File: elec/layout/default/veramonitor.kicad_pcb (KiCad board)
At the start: 2 copper layers, 55 parts, among them J1 ?, U1 ?, U10 ?, U11 ?, U12 ?, U13 ?, U14 ?, U15 ?, U16 ?, U17 ?, U18 ?, U19 ?, U2 ?, U20 ?, U21 ?, U22 ?, U23 ?, U24 ?, U25 ?, U26 ?, U3 ?, U4 ?, U5 ?, U6 ?, U7 ?, U8 ?, U9 ?

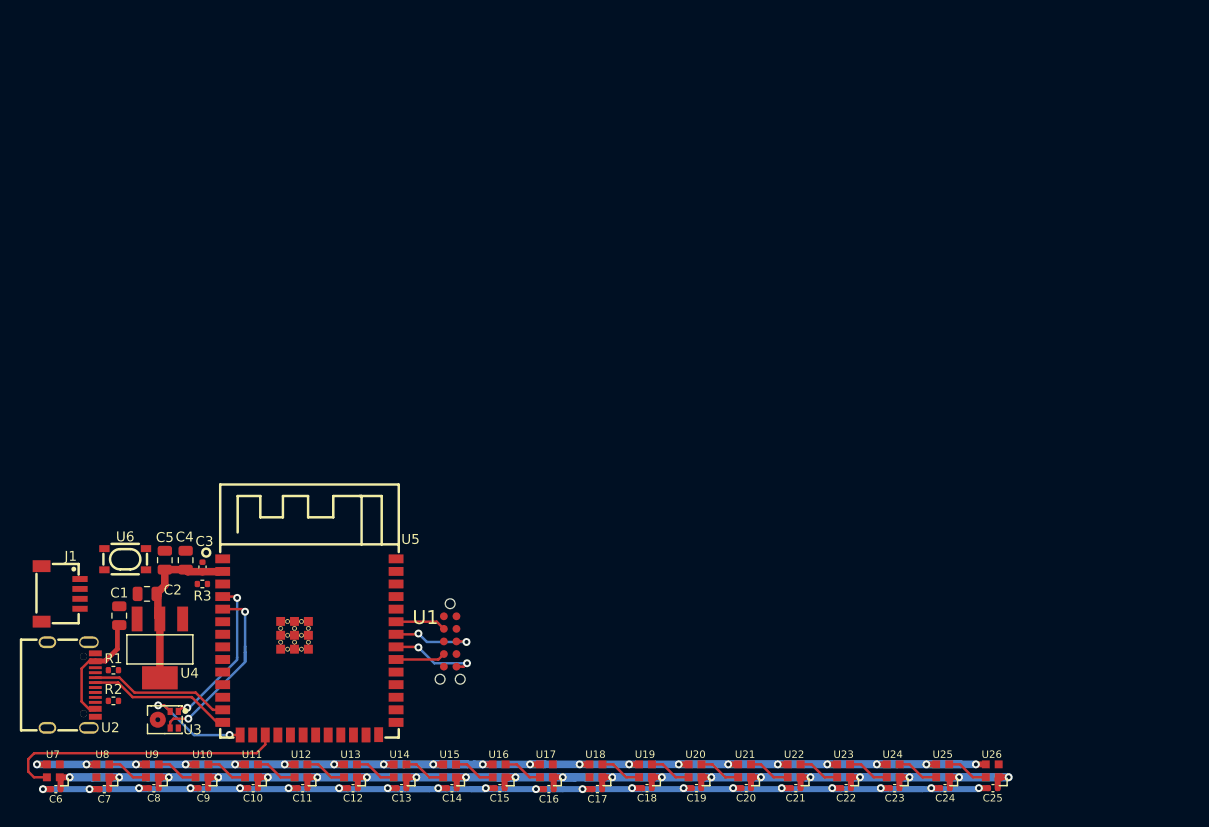
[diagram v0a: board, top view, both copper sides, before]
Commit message: eod 10/30
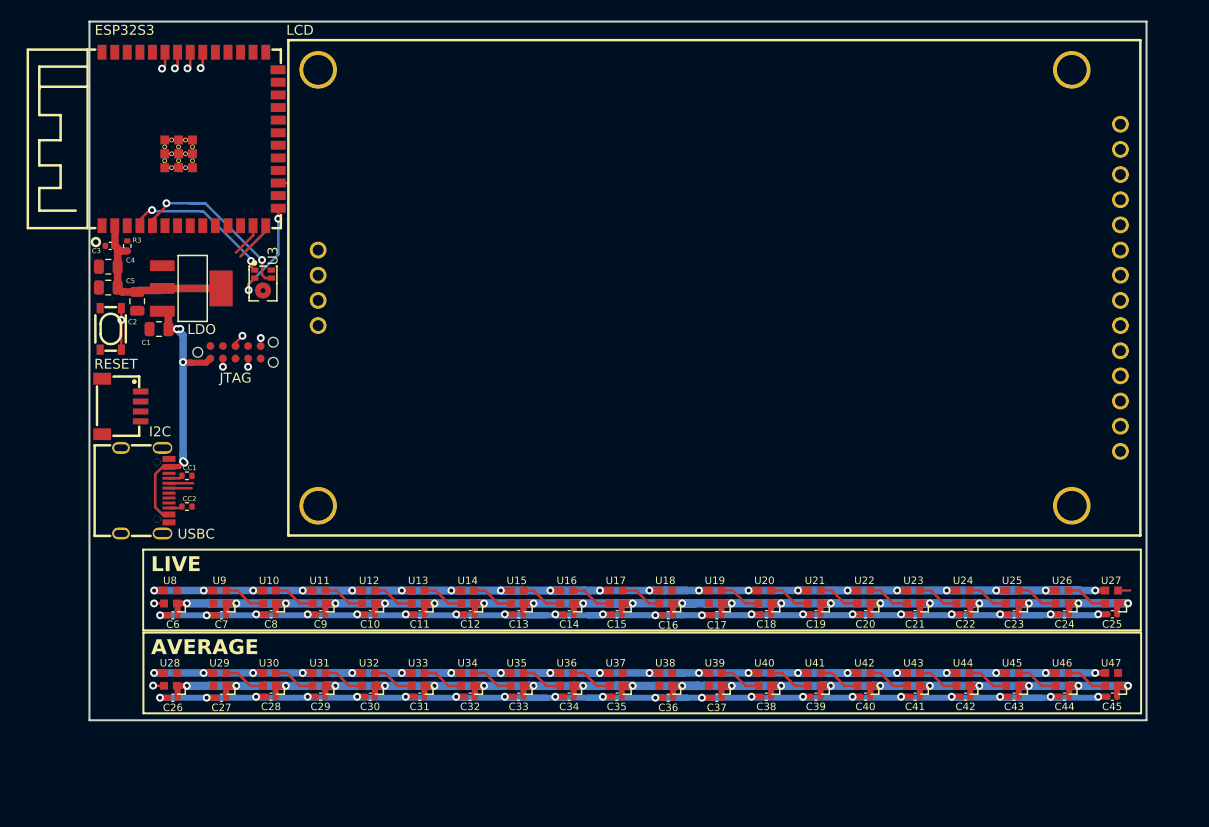
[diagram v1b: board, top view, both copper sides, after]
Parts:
- added C26: 16V 100nF X7R ±10% 0402 Multilayer Ceramic Capacitors MLCC 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, lib:C0402, F.Cu at (48.8, 135.2)
- added C27: 16V 100nF X7R ±10% 0402 Multilayer Ceramic Capacitors MLCC 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, lib:C0402, F.Cu at (53.7, 135.2)
- added C28: 16V 100nF X7R ±10% 0402 Multilayer Ceramic Capacitors MLCC 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, lib:C0402, F.Cu at (58.7, 135.1)
- added C29: 16V 100nF X7R ±10% 0402 Multilayer Ceramic Capacitors MLCC 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, lib:C0402, F.Cu at (63.7, 135.1)
- added C30: 16V 100nF X7R ±10% 0402 Multilayer Ceramic Capacitors MLCC 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, lib:C0402, F.Cu at (68.7, 135.1)
- added C31: 16V 100nF X7R ±10% 0402 Multilayer Ceramic Capacitors MLCC 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, lib:C0402, F.Cu at (73.7, 135.1)
- added C32: 16V 100nF X7R ±10% 0402 Multilayer Ceramic Capacitors MLCC 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, lib:C0402, F.Cu at (78.8, 135.1)
- added C33: 16V 100nF X7R ±10% 0402 Multilayer Ceramic Capacitors MLCC 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, lib:C0402, F.Cu at (83.7, 135.1)
- added C34: 16V 100nF X7R ±10% 0402 Multilayer Ceramic Capacitors MLCC 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, lib:C0402, F.Cu at (88.8, 135.1)
- added C35: 16V 100nF X7R ±10% 0402 Multilayer Ceramic Capacitors MLCC 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, lib:C0402, F.Cu at (93.6, 135.1)
- added C36: 16V 100nF X7R ±10% 0402 Multilayer Ceramic Capacitors MLCC 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, lib:C0402, F.Cu at (98.8, 135.2)
- added C37: 16V 100nF X7R ±10% 0402 Multilayer Ceramic Capacitors MLCC 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, lib:C0402, F.Cu at (103.7, 135.2)
- added C38: 16V 100nF X7R ±10% 0402 Multilayer Ceramic Capacitors MLCC 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, lib:C0402, F.Cu at (108.7, 135.1)
- added C39: 16V 100nF X7R ±10% 0402 Multilayer Ceramic Capacitors MLCC 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, lib:C0402, F.Cu at (113.7, 135.1)
- added C40: 16V 100nF X7R ±10% 0402 Multilayer Ceramic Capacitors MLCC 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, lib:C0402, F.Cu at (118.7, 135.1)
- added C41: 16V 100nF X7R ±10% 0402 Multilayer Ceramic Capacitors MLCC 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, lib:C0402, F.Cu at (123.7, 135.1)
- added C42: 16V 100nF X7R ±10% 0402 Multilayer Ceramic Capacitors MLCC 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, lib:C0402, F.Cu at (128.8, 135.1)
- added C43: 16V 100nF X7R ±10% 0402 Multilayer Ceramic Capacitors MLCC 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, lib:C0402, F.Cu at (133.7, 135.1)
- added C44: 16V 100nF X7R ±10% 0402 Multilayer Ceramic Capacitors MLCC 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, lib:C0402, F.Cu at (138.8, 135.1)
- added C45: 16V 100nF X7R ±10% 0402 Multilayer Ceramic Capacitors MLCC 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, lib:C0402, F.Cu at (143.6, 135.1)
- added LCD: ?, lib:COMM-TH_HS12864G18B, F.Cu at (103.9, 93.8)
- added U28: ?, lib:LED-SMD_4P-L2.0-W2.0-BR, F.Cu at (48.5, 133.4)
- added U29: ?, lib:LED-SMD_4P-L2.0-W2.0-BR, F.Cu at (53.5, 133.4)
- added U30: ?, lib:LED-SMD_4P-L2.0-W2.0-BR, F.Cu at (58.5, 133.4)
- added U31: ?, lib:LED-SMD_4P-L2.0-W2.0-BR, F.Cu at (63.5, 133.4)
- added U32: ?, lib:LED-SMD_4P-L2.0-W2.0-BR, F.Cu at (68.5, 133.4)
- added U33: ?, lib:LED-SMD_4P-L2.0-W2.0-BR, F.Cu at (73.5, 133.4)
- added U34: ?, lib:LED-SMD_4P-L2.0-W2.0-BR, F.Cu at (78.5, 133.4)
- added U35: ?, lib:LED-SMD_4P-L2.0-W2.0-BR, F.Cu at (83.5, 133.4)
- added U36: ?, lib:LED-SMD_4P-L2.0-W2.0-BR, F.Cu at (88.5, 133.4)
- added U37: ?, lib:LED-SMD_4P-L2.0-W2.0-BR, F.Cu at (93.5, 133.4)
- added U38: ?, lib:LED-SMD_4P-L2.0-W2.0-BR, F.Cu at (98.5, 133.4)
- added U39: ?, lib:LED-SMD_4P-L2.0-W2.0-BR, F.Cu at (103.5, 133.4)
- added U40: ?, lib:LED-SMD_4P-L2.0-W2.0-BR, F.Cu at (108.5, 133.4)
- added U41: ?, lib:LED-SMD_4P-L2.0-W2.0-BR, F.Cu at (113.5, 133.4)
- added U42: ?, lib:LED-SMD_4P-L2.0-W2.0-BR, F.Cu at (118.5, 133.4)
- added U43: ?, lib:LED-SMD_4P-L2.0-W2.0-BR, F.Cu at (123.5, 133.4)
- added U44: ?, lib:LED-SMD_4P-L2.0-W2.0-BR, F.Cu at (128.5, 133.4)
- added U45: ?, lib:LED-SMD_4P-L2.0-W2.0-BR, F.Cu at (133.5, 133.4)
- added U46: ?, lib:LED-SMD_4P-L2.0-W2.0-BR, F.Cu at (138.5, 133.4)
- added U47: ?, lib:LED-SMD_4P-L2.0-W2.0-BR, F.Cu at (143.5, 133.4)
- moved ESP32S3 52.7 mm to (50.5, 78.8), turned to 90 degrees
- moved U3 45.2 mm to (57.9, 93.3), turned to 0 degrees
- moved LDO 36.5 mm to (50.7, 93.9), turned to 180 degrees
- moved JTAG 36.3 mm to (55.1, 100.4), turned to 0 degrees
- moved R3 35.0 mm to (44.2, 89.6), turned to 90 degrees
- moved C3 33.7 mm to (42.5, 89.6), turned to 180 degrees
- moved C4 30.6 mm to (42.2, 91.7), turned to 180 degrees
- moved C2 29.5 mm to (45.2, 95.2), turned to -90 degrees
- moved C1 29.2 mm to (47.4, 98.0), turned to 180 degrees
- moved C5 28.1 mm to (42.2, 93.8), turned to 180 degrees
- moved RESET 23.3 mm to (42.5, 98.0), turned to -90 degrees
- moved C22 21.3 mm to (128.8, 126.8)
- moved C23 21.3 mm to (133.7, 126.8)
- moved C25 21.3 mm to (143.6, 126.8)
- moved U18 21.3 mm to (98.5, 125.0)
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- renumbered R1 to CC1, R2 to CC2, U5 to ESP32S3, J1 to I2C, U1 to JTAG, U4 to LDO, U6 to RESET, U9 to U10, U10 to U11, U11 to U12, U12 to U13, U13 to U14, U14 to U15, U15 to U16, U16 to U17, U17 to U18, U18 to U19, U19 to U20, U20 to U21, U21 to U22, U22 to U23, U23 to U24, U24 to U25, U25 to U26, U26 to U27, U7 to U8, U8 to U9, U2 to USBC
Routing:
- net gnd: track 314.7 -> 636.1 mm, vias 40 -> 80
- net vcc: track 176.0 -> 349.7 mm, vias 20 -> 45
- net led_data: track 28.9 -> 1.97 mm, vias 0 -> 1
- net dm: track 14.2 -> 5.88 mm
- net dp: track 14.5 -> 6.47 mm
- net tdo: track 9.05 -> 2.55 mm
- net tdi: track 8.60 -> 3.16 mm
- net ledrow4.led6.ic-vcc: track 0.00 -> 4.24 mm
- net ledrow4.led5.ic-vcc: track 0.00 -> 4.24 mm
- net ledrow4.led4.ic-vcc: track 0.00 -> 4.24 mm
- net ledrow4.led3.ic-vcc: track 0.00 -> 4.24 mm
- net ledrow4.led2.ic-vcc: track 0.00 -> 4.24 mm
- net ledrow3.led9.ic-vcc: track 0.00 -> 4.24 mm
- net ledrow3.led8.ic-vcc: track 0.00 -> 4.24 mm
- net ledrow3.led7.ic-vcc: track 0.00 -> 4.24 mm
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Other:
- board outline added: 106.7 x 70.5 mm
- board text added: "AVERAGE"
- board text added: "LIVE"

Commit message: finished?
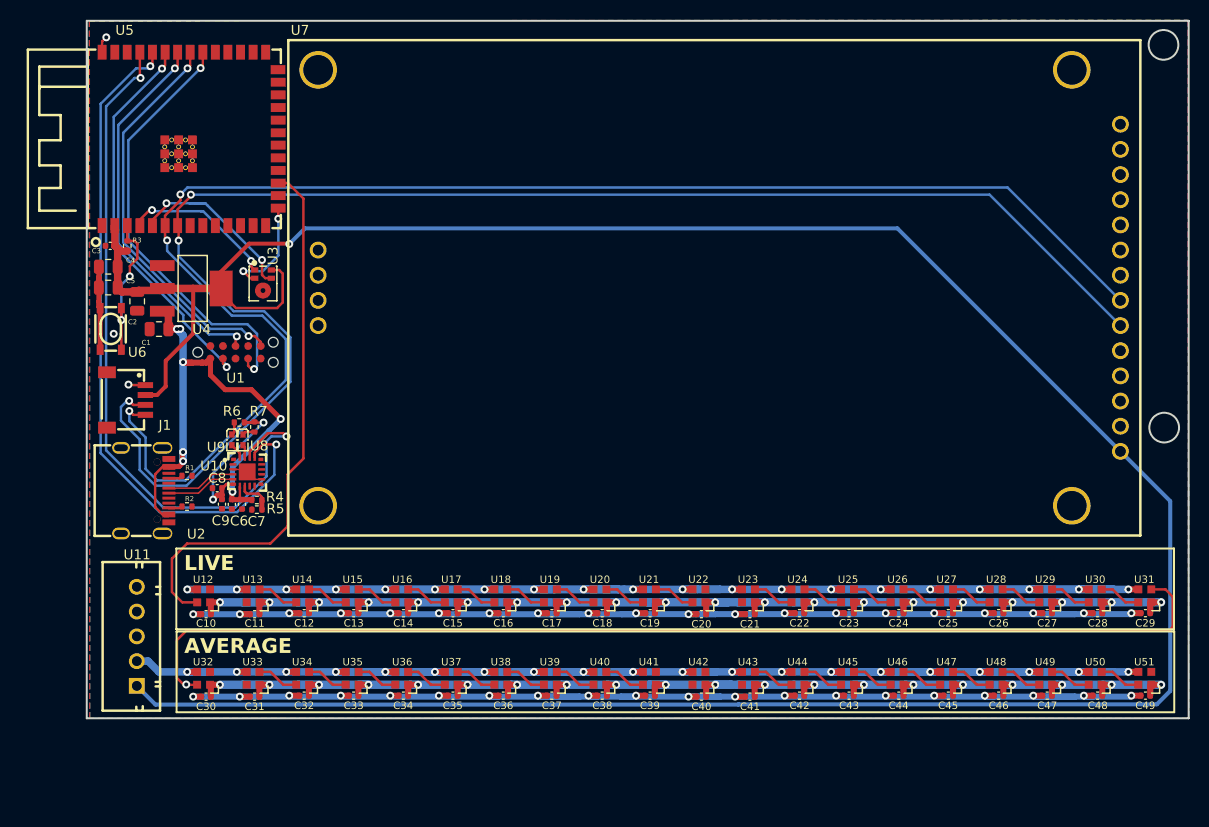
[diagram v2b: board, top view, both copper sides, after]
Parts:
- added C6: 6.3V 10uF X5R ±20% 0402 Multilayer Ceramic Capacitors MLCC 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, lib:C0402, F.Cu at (54.7, 115.7)
- added C7: 50V 10nF X7R ±10% 0402 Multilayer Ceramic Capacitors MLCC -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, lib:C0402, F.Cu at (55.8, 115.7)
- added C8: 6.3V 10uF X5R ±20% 0402 Multilayer Ceramic Capacitors MLCC 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, lib:C0402, F.Cu at (53.2, 114.1)
- added C9: 50V 10nF X7R ±10% 0402 Multilayer Ceramic Capacitors MLCC -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, lib:C0402, F.Cu at (53.7, 115.7)
- added R4: 62.5mW Thick Film Resistors 50V ±100ppm/℃ ±1% 20kΩ 0402 Chi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, lib:R0402, F.Cu at (57.2, 115.3)
- added R5: 62.5mW Thick Film Resistors 50V ±100ppm/℃ ±1% 51kΩ 0402 Chi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, lib:R0402, F.Cu at (57.2, 116.2)
- added R6: 62.5mW Thick Film Resistors 50V ±100ppm/℃ ±1% 20kΩ 0402 Chi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, lib:R0402, F.Cu at (55.5, 107.4)
- added R7: 62.5mW Thick Film Resistors 50V ±100ppm/℃ ±1% 20kΩ 0402 Chi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, lib:R0402, F.Cu at (57.0, 107.9)
- added U10: ?, lib:QFN-20_L3.0-W3.0-P0.50-BL-EP1.7_EFM8BB21F16G, F.Cu at (56.3, 112.4)
- added U11: ?, lib:CONN-TH_5P-P2.50_XH-5A_C2318, F.Cu at (45.1, 129.0)
- added U8: ?, lib:LED0402-RD, F.Cu at (55.9, 109.2)
- added U9: ?, lib:LED0402-RD, F.Cu at (54.7, 109.2)
- C1, C2, C4, C5: value 25V 10uF X5R ±10% 0805 Multilayer Ceramic Capacitors MLCC - SMD/SMT ROHS -> 25V 10uF X5R ±10% 0805 Multilayer Ceramic Capacitors MLCC - SMD/SMT ROHS
- C3: value 16V 100nF X7R ±10% 0402 Multilayer Ceramic Capacitors MLCC - SMD/SMT ROHS -> 16V 100nF X7R ±10% 0402 Multilayer Ceramic Capacitors MLCC - SMD/SMT ROHS
- R1: renamed from CC1; value 62.5mW Thick Film Resistors 50V ±100ppm/℃ ±1% 5.1kΩ 0402 Chip Resistor - Surface Mount ROHS -> 62.5mW Thick Film Resistors 50V ±100ppm/℃ ±1% 5.1kΩ 0402 Chip Resistor - Surface Mount ROHS
- R2: renamed from CC2; value 62.5mW Thick Film Resistors 50V ±100ppm/℃ ±1% 5.1kΩ 0402 Chip Resistor - Surface Mount ROHS -> 62.5mW Thick Film Resistors 50V ±100ppm/℃ ±1% 5.1kΩ 0402 Chip Resistor - Surface Mount ROHS
- R3: value 62.5mW Thick Film Resistors 50V ±100ppm/℃ ±1% 10kΩ 0402 Chip Resistor - Surface Mount ROHS -> 62.5mW Thick Film Resistors 50V ±100ppm/℃ ±1% 10kΩ 0402 Chip Resistor - Surface Mount ROHS
- moved C34 3.35 mm to (72.0, 135.0)
- moved C35 3.35 mm to (77.0, 135.0)
- moved C44 3.35 mm to (122.0, 135.0)
- moved C45 3.35 mm to (127.0, 135.0)
- moved C24 3.35 mm to (122.0, 126.7)
- moved C25 3.35 mm to (127.0, 126.7)
- moved C13 3.35 mm to (67.0, 126.7)
- moved C32 3.35 mm to (62.0, 135.0)
- moved U35 3.35 mm to (66.9, 133.3)
- moved C31 3.35 mm to (57.0, 135.1)
- moved C12 3.35 mm to (62.0, 126.7)
- moved C14 3.35 mm to (72.0, 126.7)
- moved C15 3.35 mm to (77.0, 126.7)
- moved C16 3.35 mm to (82.1, 126.7)
- moved C17 3.35 mm to (87.0, 126.7)
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- renumbered C6 to C10, C7 to C11, C8 to C12, C9 to C13, C10 to C14, C11 to C15, C12 to C16, C13 to C17, C14 to C18, C15 to C19, C16 to C20, C17 to C21, C18 to C22, C19 to C23, C20 to C24, C21 to C25, C22 to C26, C23 to C27, C24 to C28, C25 to C29, C26 to C30, C27 to C31, C28 to C32, C29 to C33, C30 to C34, C31 to C35, C32 to C36, C33 to C37, C34 to C38, C35 to C39, C36 to C40, C37 to C41, C38 to C42, C39 to C43, C40 to C44, C41 to C45, C42 to C46, C43 to C47, C44 to C48, C45 to C49, I2C to J1, JTAG to U1, U8 to U12, U9 to U13, U10 to U14, U11 to U15, U12 to U16, U13 to U17, U14 to U18, U15 to U19, USBC to U2, U16 to U20, U17 to U21, U18 to U22, U19 to U23, U20 to U24, U21 to U25, U22 to U26, U23 to U27, U24 to U28, U25 to U29, U26 to U30, U27 to U31, U28 to U32, U29 to U33, U30 to U34, U31 to U35, U32 to U36, U33 to U37, U34 to U38, U35 to U39, LDO to U4, U36 to U40, U37 to U41, U38 to U42, U39 to U43, U40 to U44, U41 to U45, U42 to U46, U43 to U47, U44 to U48, U45 to U49, ESP32S3 to U5, U46 to U50, U47 to U51, RESET to U6, LCD to U7
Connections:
- net nc renamed lcd-nc
- J1 pad 1: i2c_connector-gnd -> gnd
- J1 pad 2: i2c_connector-vcc -> vcc-1
- U5 pad 13: dm -> io19
- U5 pad 14: dp -> io20
- U5 pad 36: rxd0 -> rx
- U5 pad 37: txd0 -> tx
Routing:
- net vcc-1: track 18.7 -> 279.6 mm, vias 0 -> 1
- net sda: track 0.00 -> 155.5 mm, vias 0 -> 3
- net scl: track 0.00 -> 153.3 mm, vias 0 -> 3
- net ledrow2-dout: track 2.34 -> 112.8 mm
- net tx: track 0.00 -> 72.9 mm, vias 0 -> 2
- net rx: track 0.00 -> 71.1 mm, vias 0 -> 2
- net led_data: track 1.97 -> 56.3 mm, vias 1 -> 0
- net tck: track 2.52 -> 44.2 mm
- net tdo: track 2.55 -> 40.4 mm
- net tms: track 2.83 -> 39.9 mm
- net tdi: track 3.16 -> 38.8 mm
- net vcc: track 349.7 -> 376.8 mm, vias 45 -> 47
- net gnd: track 636.1 -> 661.7 mm, vias 80 -> 83
- net vdd: track 0.00 -> 16.2 mm, vias 0 -> 2
- net en: track 4.20 -> 15.3 mm, vias 1 -> 2
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- added copper zone on B.Cu, net gnd
- added copper zone on F.Cu, net gnd
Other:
- board size 106.7 x 70.5 mm -> 111.2 x 70.4 mm
